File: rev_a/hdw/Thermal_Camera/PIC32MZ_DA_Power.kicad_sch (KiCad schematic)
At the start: 19 parts

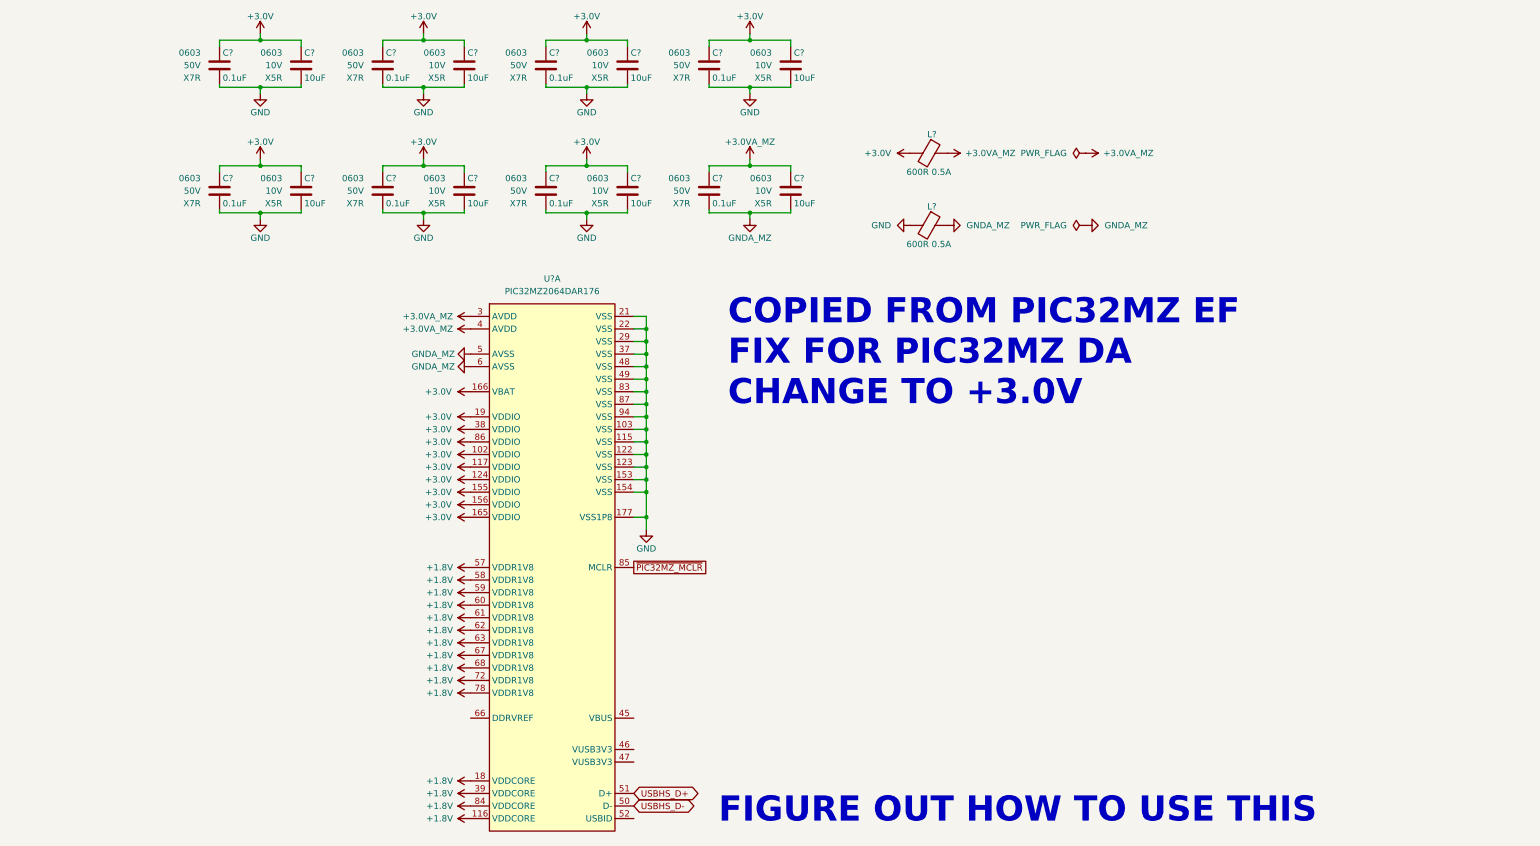
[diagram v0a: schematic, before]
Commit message: added PIC32 bypass, SD card load switch, other random junk
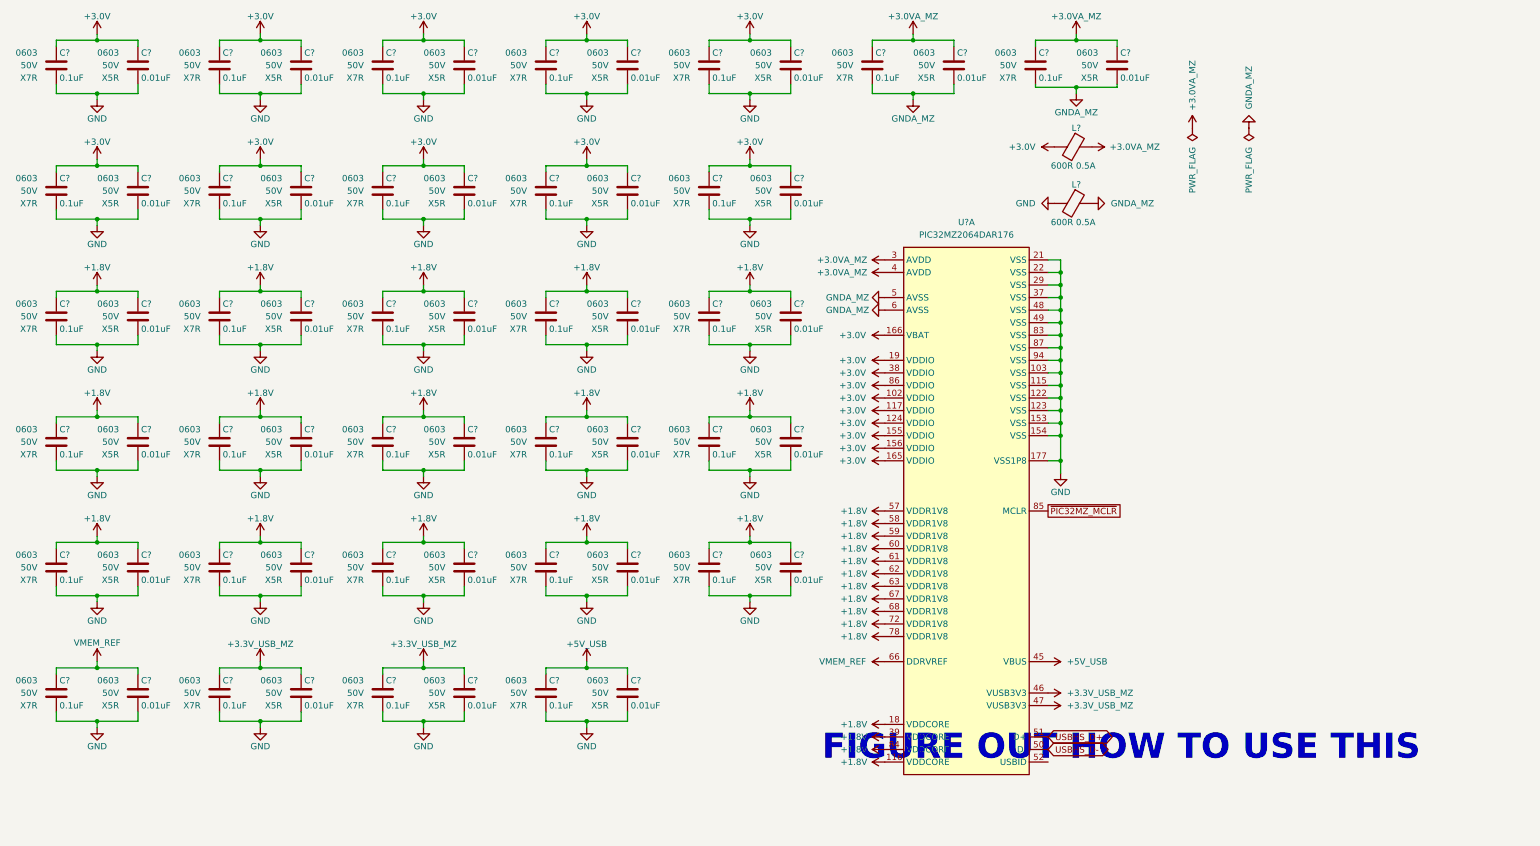
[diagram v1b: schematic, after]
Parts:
- removed C? (x7): 10uF, Capacitors_SMD:C_0603, symbol Custom_Library:C_Custom
- added C? (x23): 0.1uF, Capacitors_SMD:C_0603, symbol Custom_Library:C_Custom
- added C? (x30): 0.01uF, Capacitors_SMD:C_0603, symbol Custom_Library:C_Custom
- C?: value 10uF -> 0.01uF; Digi-Key PN 1276-1871-1-ND -> (none); Voltage 10V -> 50V
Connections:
- net +1.8V: now also C?.1, C?.1, C?.1, C?.1, C?.1, C?.1, C?.1, C?.1, C?.1, C?.1, C?.1, C?.1, C?.1, C?.1, C?.1, C?.1, C?.1, C?.1, C?.1, C?.1, C?.1, C?.1, C?.1, C?.1, C?.1, C?.1, C?.1, C?.1, C?.1, C?.1
- net +3.0V: now also C?.1, C?.1, C?.1, C?.1, C?.1, C?.1, C?.1, C?.1, C?.1, C?.1, C?.1, C?.1
- net +3.0VA_MZ: now also C?.1, C?.1, C?.1
- net GND: now also C?.2, C?.2, C?.2, C?.2, C?.2, C?.2, C?.2, C?.2, C?.2, C?.2, C?.2, C?.2, C?.2, C?.2, C?.2, C?.2, C?.2, C?.2, C?.2, C?.2, C?.2, C?.2, C?.2, C?.2, C?.2, C?.2, C?.2, C?.2, C?.2, C?.2, C?.2, C?.2, C?.2, C?.2, C?.2, C?.2, C?.2, C?.2, C?.2, C?.2, C?.2, C?.2, C?.2, C?.2, C?.2, C?.2, C?.2, C?.2, C?.2, C?.2
- net GNDA_MZ: now also C?.2, C?.2, C?.2
- net +5V_USB: now reaches U?.45 (VBUS)
- net +5V_USB: now also C?.1, C?.1
- net +3.3V_USB_MZ: now reaches U?.46 (VUSB3V3)
- net +3.3V_USB_MZ: now also U?.47 (VUSB3V3), C?.1, C?.1, C?.1, C?.1
- net VMEM_REF: now reaches U?.66 (DDRVREF)
- net VMEM_REF: now also C?.1, C?.1
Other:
- note removed: "COPIED FROM PIC32MZ EF FIX FOR PIC32MZ DA CHANGE TO +3.0V"
- moved on the sheet: C?, L?, U?A
